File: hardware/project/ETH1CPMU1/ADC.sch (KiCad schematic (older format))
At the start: 4 parts, among them U1001 INA159, U1002 INA159, U1003 INA159, U1004 INA159

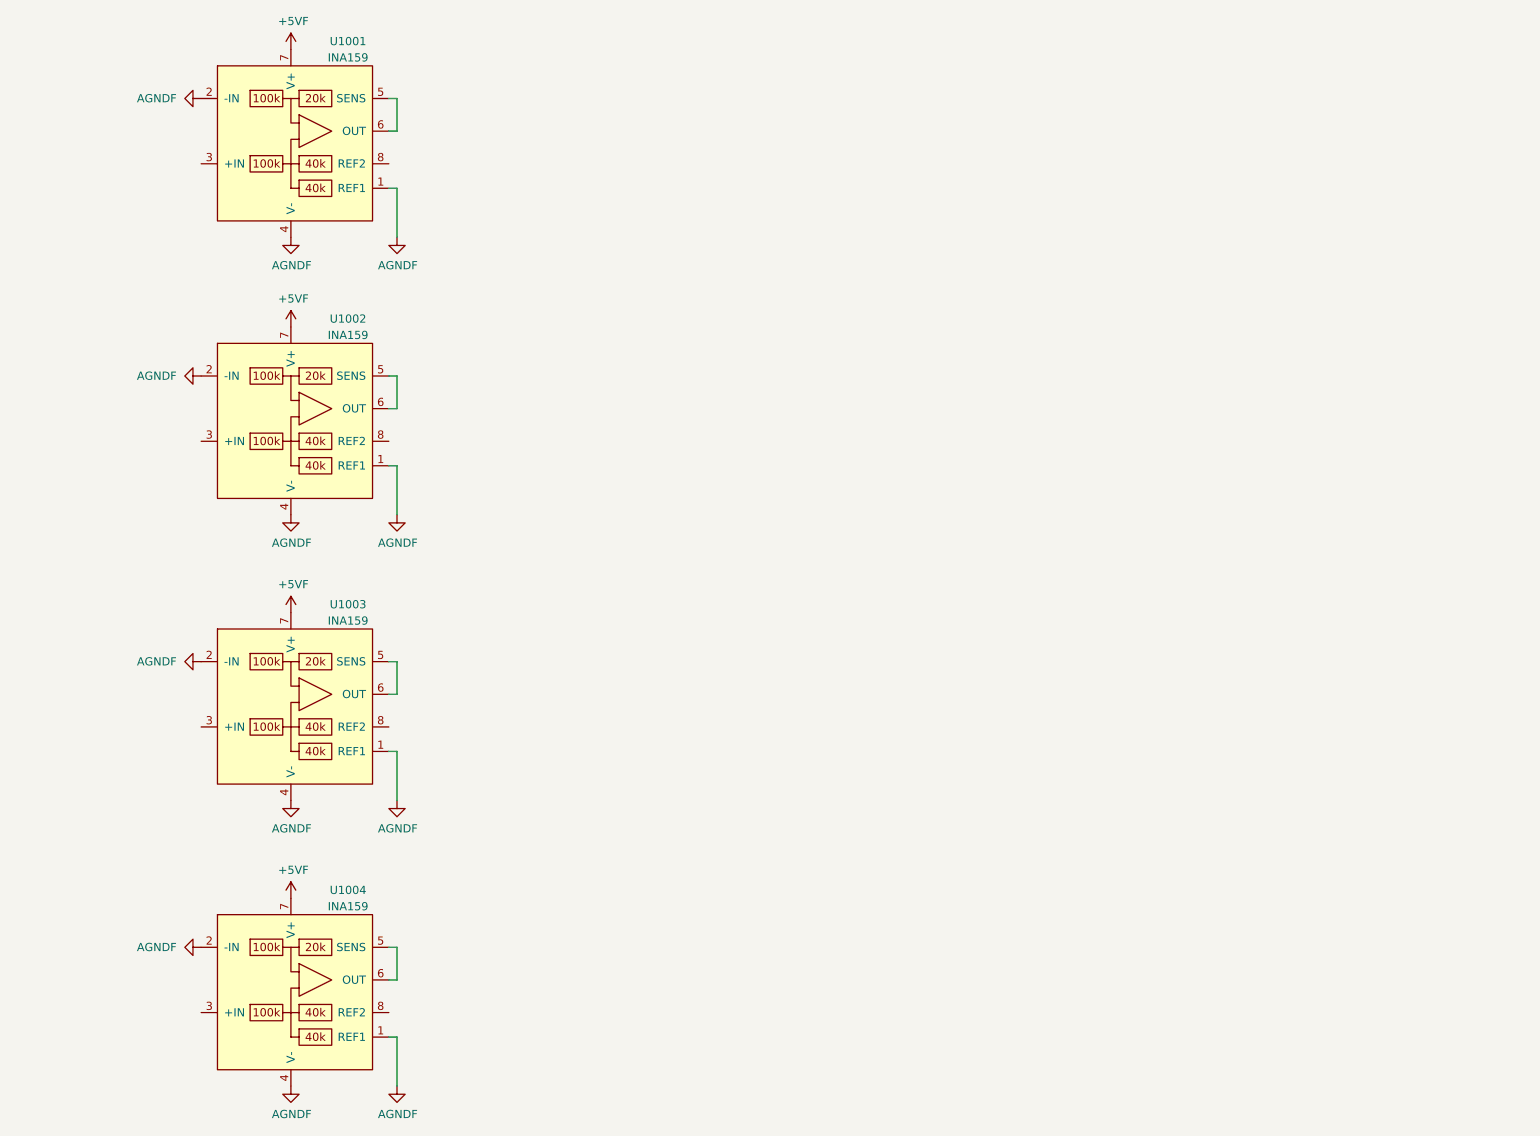
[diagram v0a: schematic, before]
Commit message: Schematic design
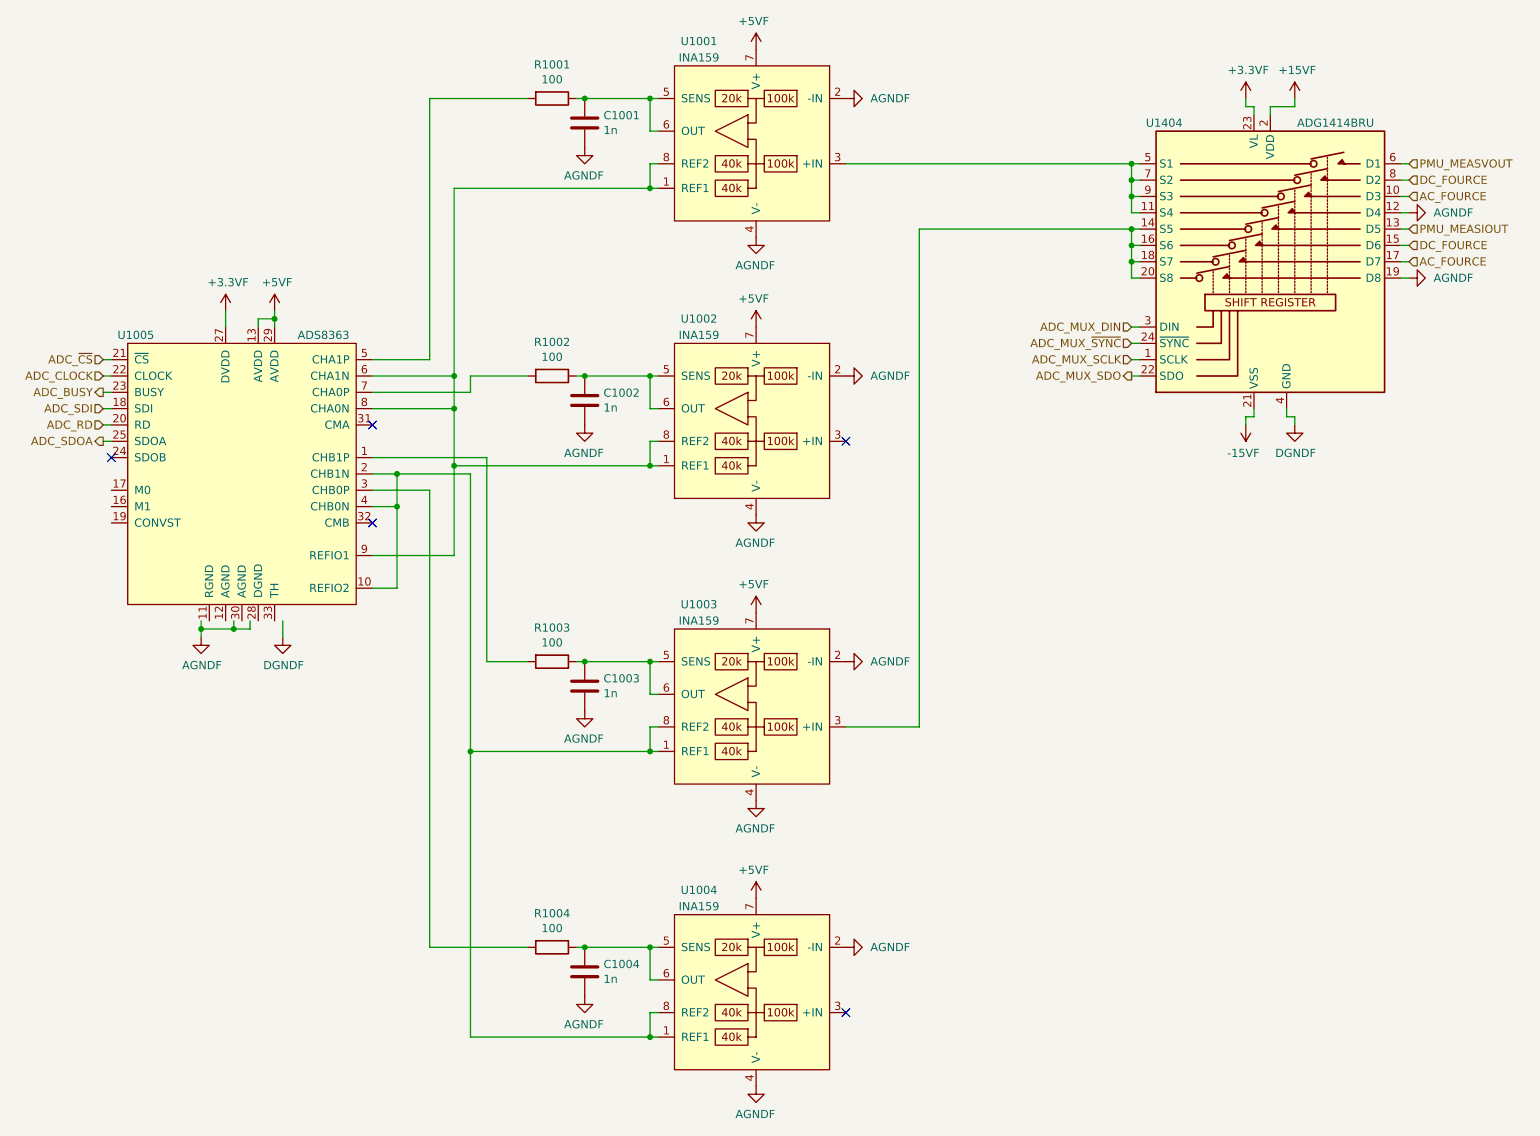
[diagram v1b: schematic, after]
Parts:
- added C1001, C1002, C1003, C1004: 1n, symbol Device:C
- added R1001, R1002, R1003, R1004: 100, symbol Device:R
- added U1005: ADS8363, symbol ETH1CPMU1:ADS8363
- added U1404: ADG1414BRU, Package_SO:TSSOP-24_4.4x7.8mm_P0.65mm, symbol Analog_Switch:ADG1414BRU
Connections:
- net labels added: +15VF, +3.3VF, -15VF, AC_FOURCE, ADC_BUSY, ADC_CLOCK, ADC_MUX_DIN, ADC_MUX_SCLK, ADC_MUX_SDO, ADC_MUX_~SYNC, ADC_RD, ADC_SDI, ADC_SDOA, ADC_~CS, DC_FOURCE, DGNDF, PMU_MEASIOUT, PMU_MEASVOUT
- wire segments 20 -> 123
- no-connect marks 0 -> 5
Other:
- moved on the sheet: U1001, U1002, U1003, U1004
